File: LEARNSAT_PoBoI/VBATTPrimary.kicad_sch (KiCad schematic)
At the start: 17 parts, among them Q12 SI7164DP-T1-GE3, Q13 SI5418DU-T1-GE3, U27 INA219AIDCNR, U29 LTC4231IUD-2#TRPBF

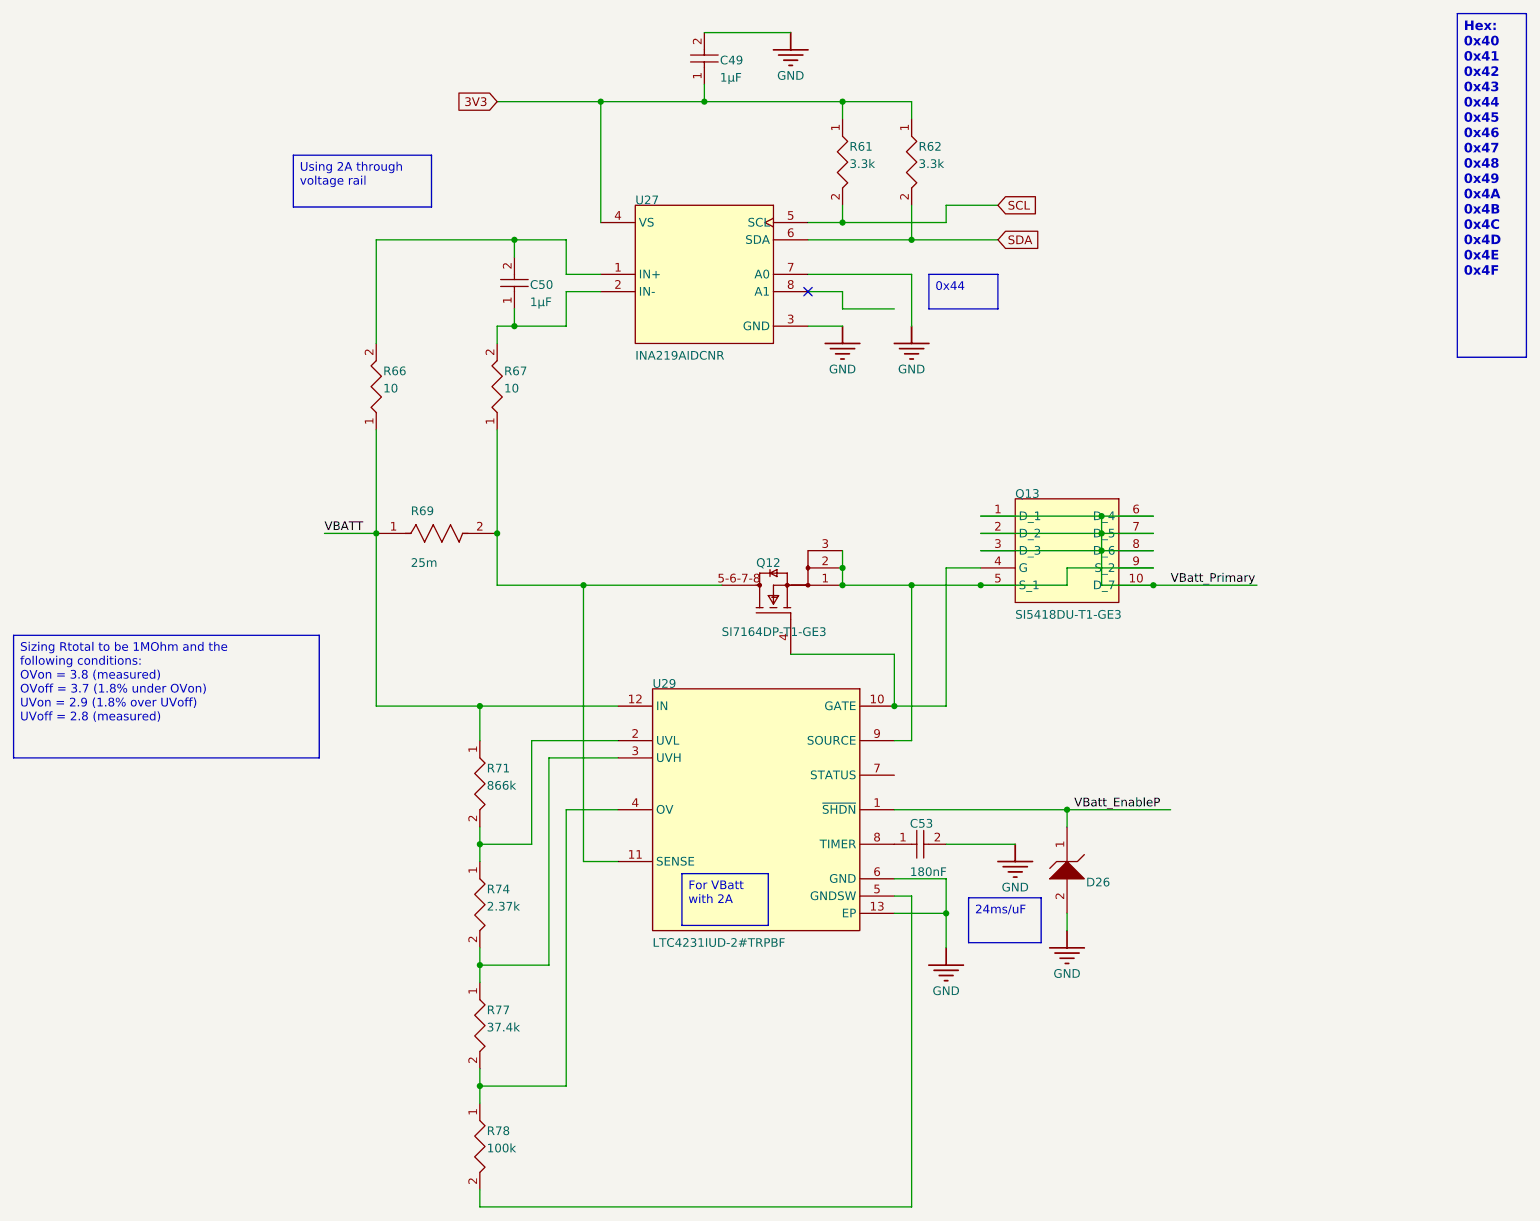
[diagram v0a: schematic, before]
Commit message: Added footprints
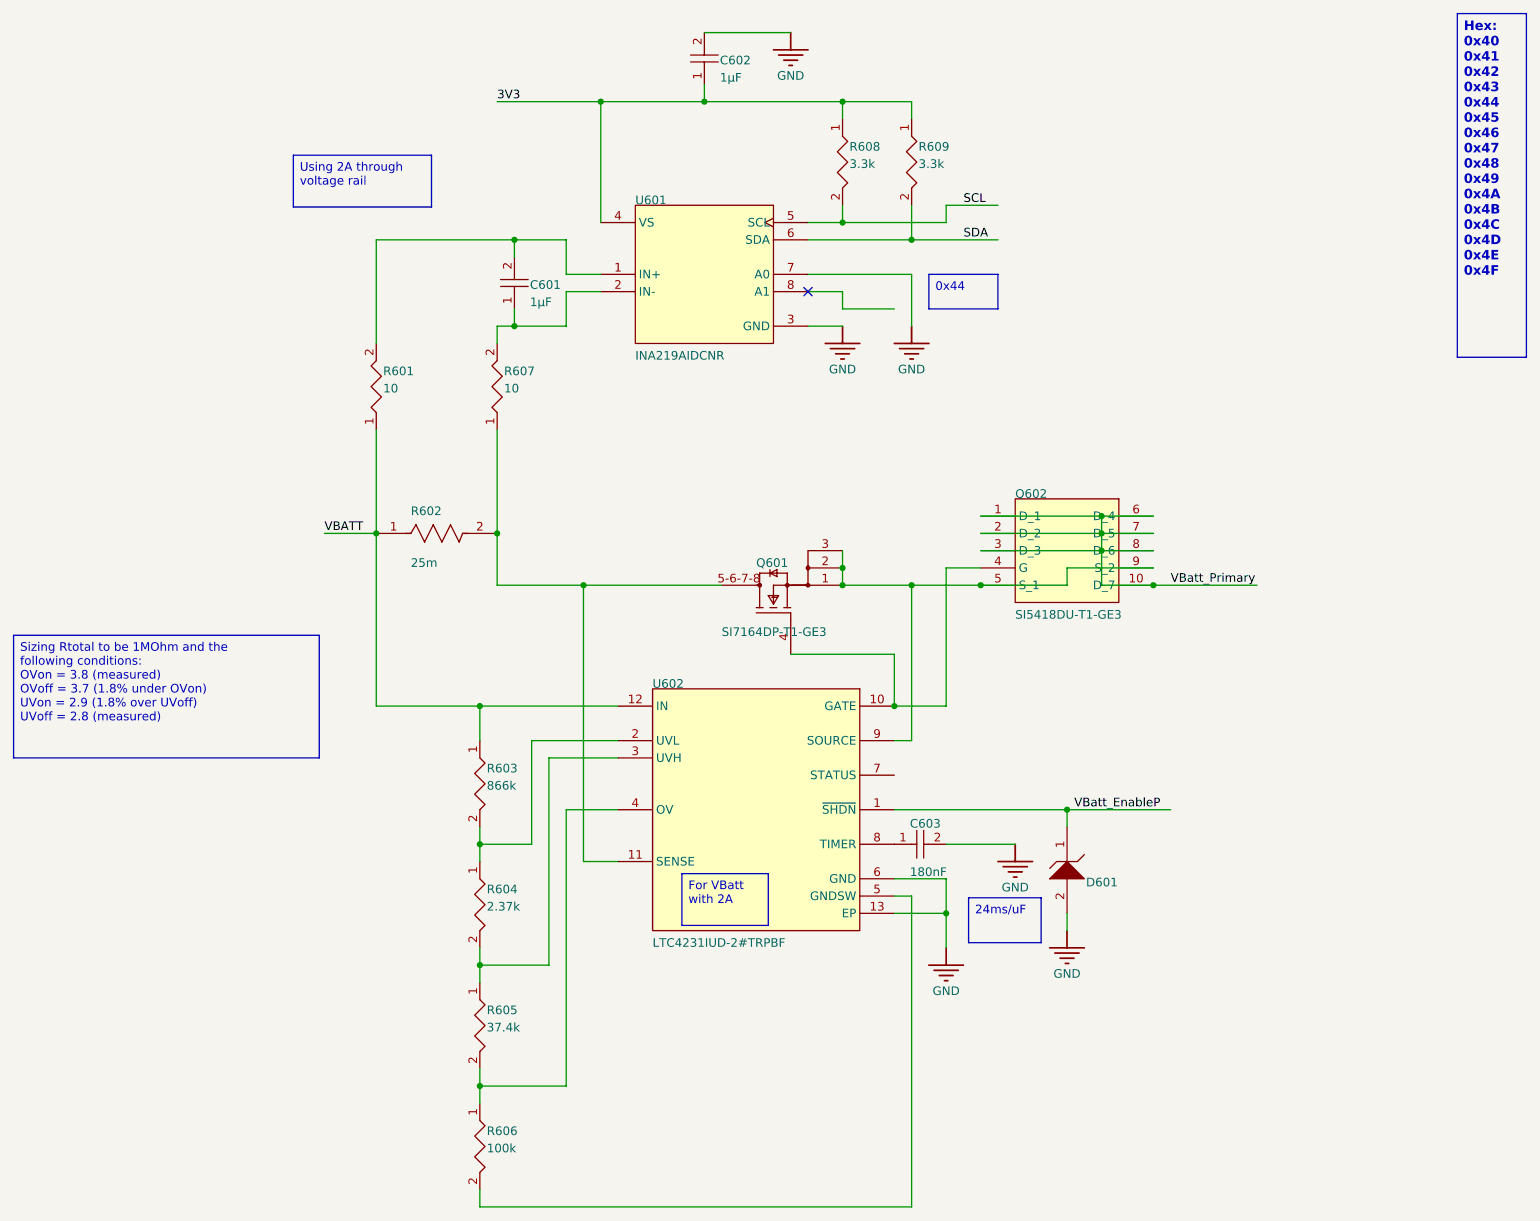
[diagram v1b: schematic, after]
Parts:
- C601: renamed from C50; footprint CAPC1608X90X40LL10T20 -> Capacitor_SMD:C_0603_1608Metric
- C602: renamed from C49; footprint CAPC1608X90X35ML15T15 -> Capacitor_SMD:C_0603_1608Metric
- C603: renamed from C53; footprint FP-C0805C-DN-IPC_A -> Capacitor_SMD:C_0805_2012Metric
- D601: renamed from D26; footprint ONSC-SOD-323-2-477-02_V -> Diode_SMD:D_SOD-323
- Q601: renamed from Q12; footprint Vishay_S17-0173-SINGLE_MFG -> Package_SO:Vishay_PowerPAK_1212-8_Single
- Q602: renamed from Q13; footprint SI5418DU-T1-GE3-Footprint-1 -> Package_SO:Vishay_PowerPAK_1212-8_Single
- R601: renamed from R66; footprint RESC0402(1005)_L -> Resistor_SMD:R_0402_1005Metric
- R602: renamed from R69; footprint FP-CSR1206-IPC_C -> Resistor_SMD:R_1206_3216Metric
- R603: renamed from R71; footprint RESC0603X26X15NL03T05 -> Resistor_SMD:R_0603_1608Metric
- R604: renamed from R74; footprint RESC0402(1005)_L -> Resistor_SMD:R_0402_1005Metric
- R605: renamed from R77; footprint FP-CR0603-IPC_A -> Resistor_SMD:R_0603_1608Metric
- R606: renamed from R78; footprint RESC1005X40X25ML05T05 -> Resistor_SMD:R_0402_1005Metric
- R607: renamed from R67; footprint RESC0402(1005)_L -> Resistor_SMD:R_0402_1005Metric
- R608: renamed from R61; footprint FP-CRCW1210-e3-IPC_C -> Resistor_SMD:R_1210_3225Metric
- R609: renamed from R62; footprint FP-CRCW1210-e3-IPC_C -> Resistor_SMD:R_1210_3225Metric
- U601: renamed from U27; footprint FP-DCN0008A-IPC_A -> INA219AIDCNR:SOT65P280X145-8N
- U602: renamed from U29; footprint FP-UD-12-05-08-1855-IPC_A -> LTC4231IUD-2_TRPBF:QFN50P300X300X80-13N

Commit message: Add files via upload
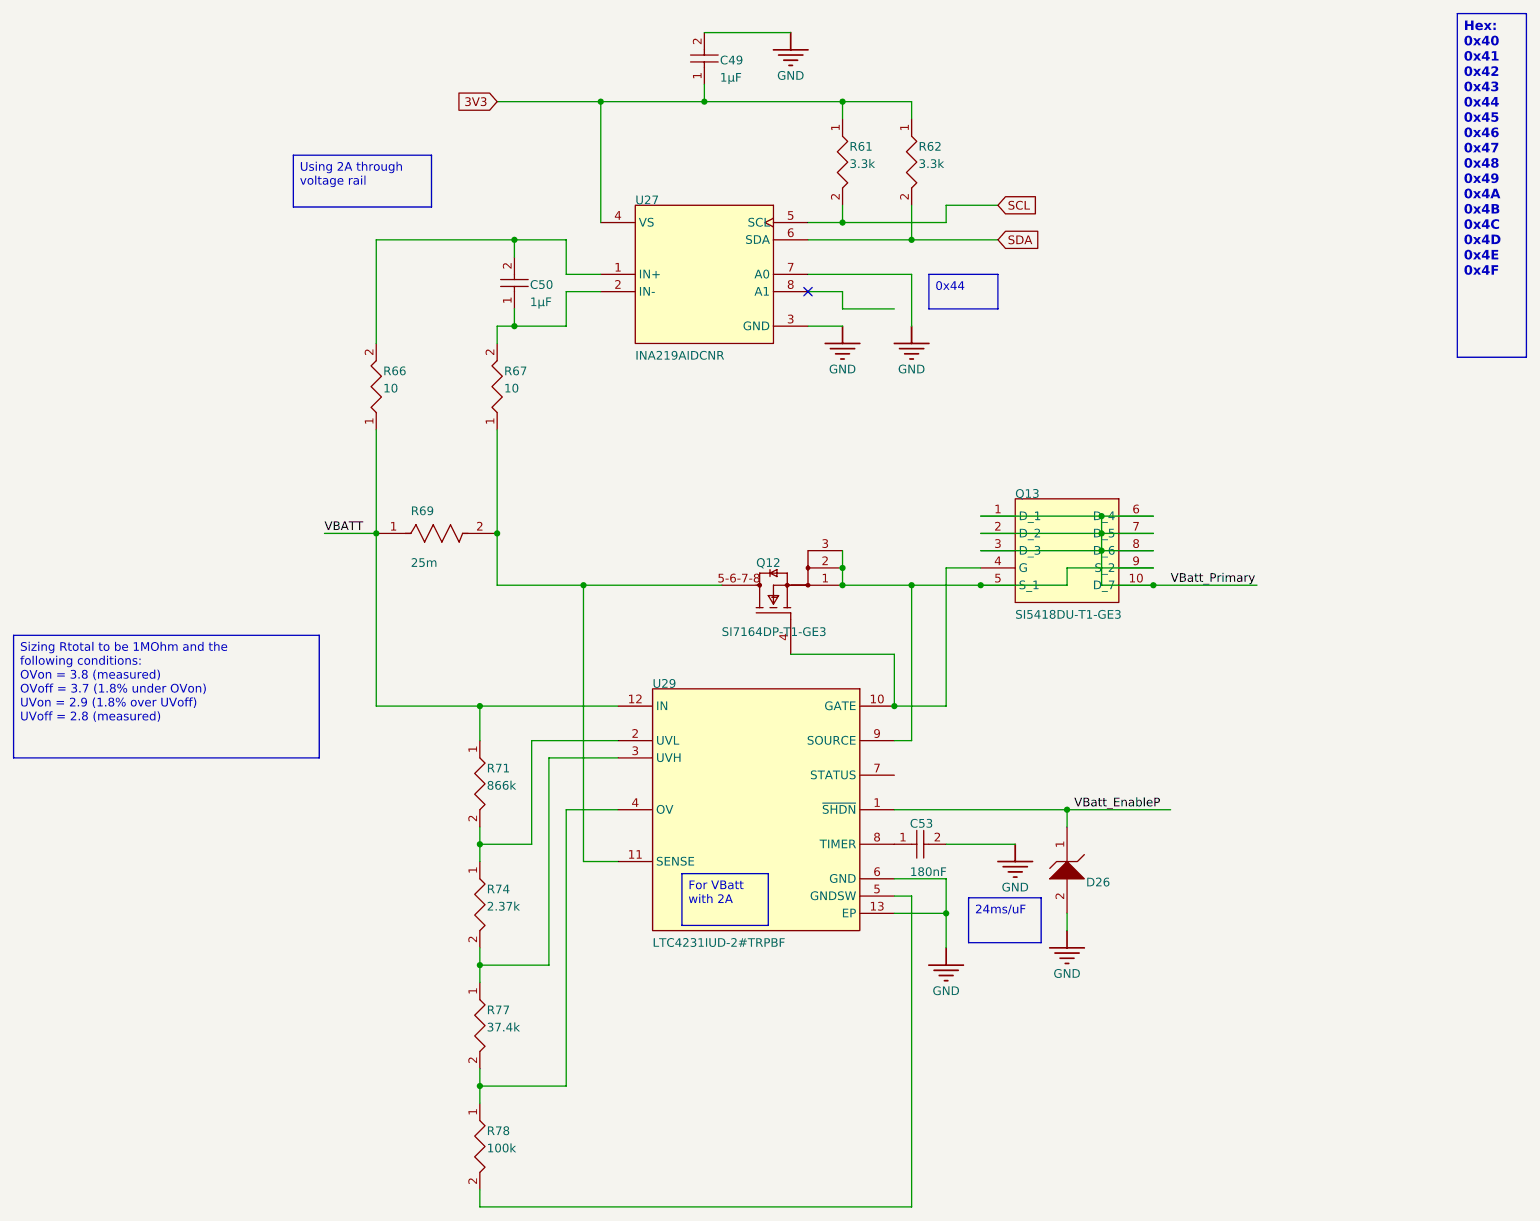
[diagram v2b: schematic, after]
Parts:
- C49: renamed from C602; footprint Capacitor_SMD:C_0603_1608Metric -> CAPC1608X90X35ML15T15
- C50: renamed from C601; footprint Capacitor_SMD:C_0603_1608Metric -> CAPC1608X90X40LL10T20
- C53: renamed from C603; footprint Capacitor_SMD:C_0805_2012Metric -> FP-C0805C-DN-IPC_A
- D26: renamed from D601; footprint Diode_SMD:D_SOD-323 -> ONSC-SOD-323-2-477-02_V
- Q12: renamed from Q601; footprint Package_SO:Vishay_PowerPAK_1212-8_Single -> Vishay_S17-0173-SINGLE_MFG
- Q13: renamed from Q602; footprint Package_SO:Vishay_PowerPAK_1212-8_Single -> SI5418DU-T1-GE3-Footprint-1
- R61: renamed from R608; footprint Resistor_SMD:R_1210_3225Metric -> FP-CRCW1210-e3-IPC_C
- R62: renamed from R609; footprint Resistor_SMD:R_1210_3225Metric -> FP-CRCW1210-e3-IPC_C
- R66: renamed from R601; footprint Resistor_SMD:R_0402_1005Metric -> RESC0402(1005)_L
- R67: renamed from R607; footprint Resistor_SMD:R_0402_1005Metric -> RESC0402(1005)_L
- R69: renamed from R602; footprint Resistor_SMD:R_1206_3216Metric -> FP-CSR1206-IPC_C
- R71: renamed from R603; footprint Resistor_SMD:R_0603_1608Metric -> RESC0603X26X15NL03T05
- R74: renamed from R604; footprint Resistor_SMD:R_0402_1005Metric -> RESC0402(1005)_L
- R77: renamed from R605; footprint Resistor_SMD:R_0603_1608Metric -> FP-CR0603-IPC_A
- R78: renamed from R606; footprint Resistor_SMD:R_0402_1005Metric -> RESC1005X40X25ML05T05
- U27: renamed from U601; footprint INA219AIDCNR:SOT65P280X145-8N -> FP-DCN0008A-IPC_A
- U29: renamed from U602; footprint LTC4231IUD-2_TRPBF:QFN50P300X300X80-13N -> FP-UD-12-05-08-1855-IPC_A
